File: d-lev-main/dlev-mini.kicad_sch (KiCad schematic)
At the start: 41 parts, among them J1 S6B-PH-SM4-TB, J2 S8B-PH-SM4-TB, J3 S8B-PH-SM4-TB, J4 S12B-PH-SM4-TB, U3 AMS1117-3.3

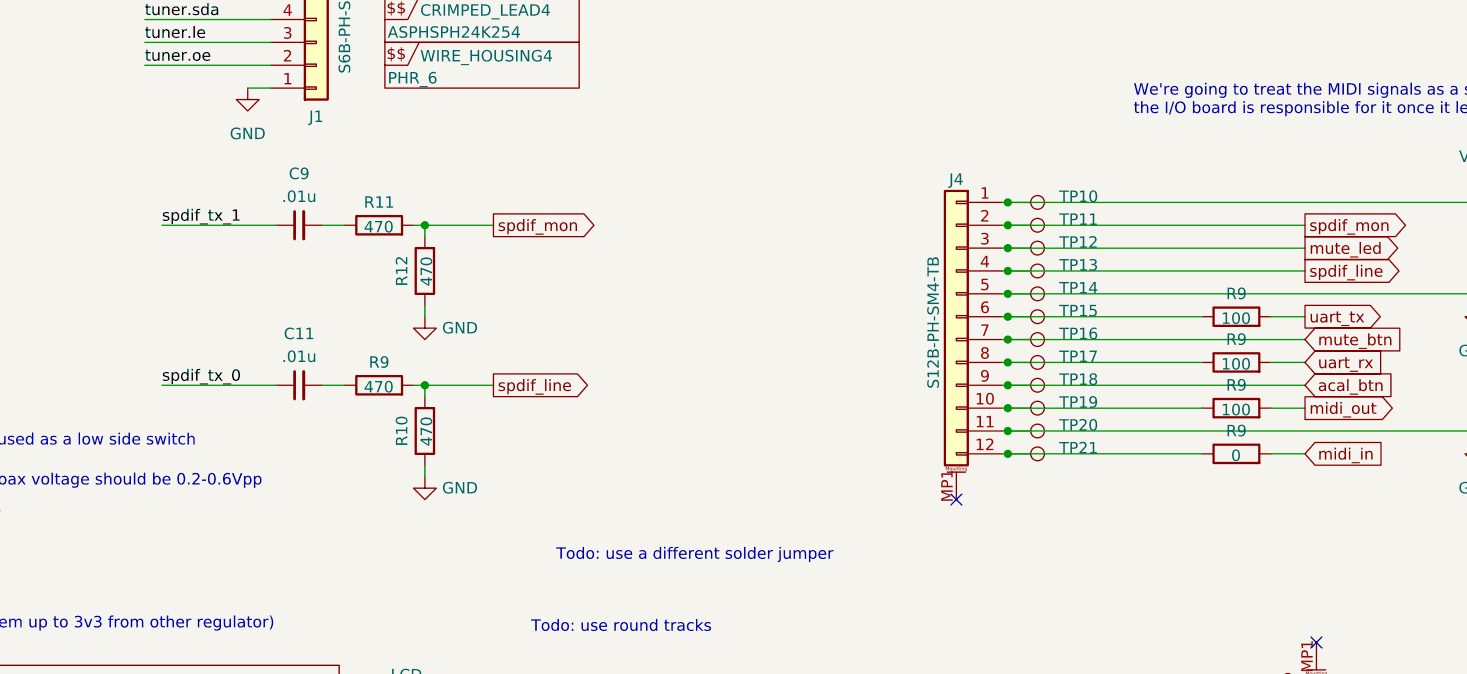
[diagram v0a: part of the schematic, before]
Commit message: many board updates
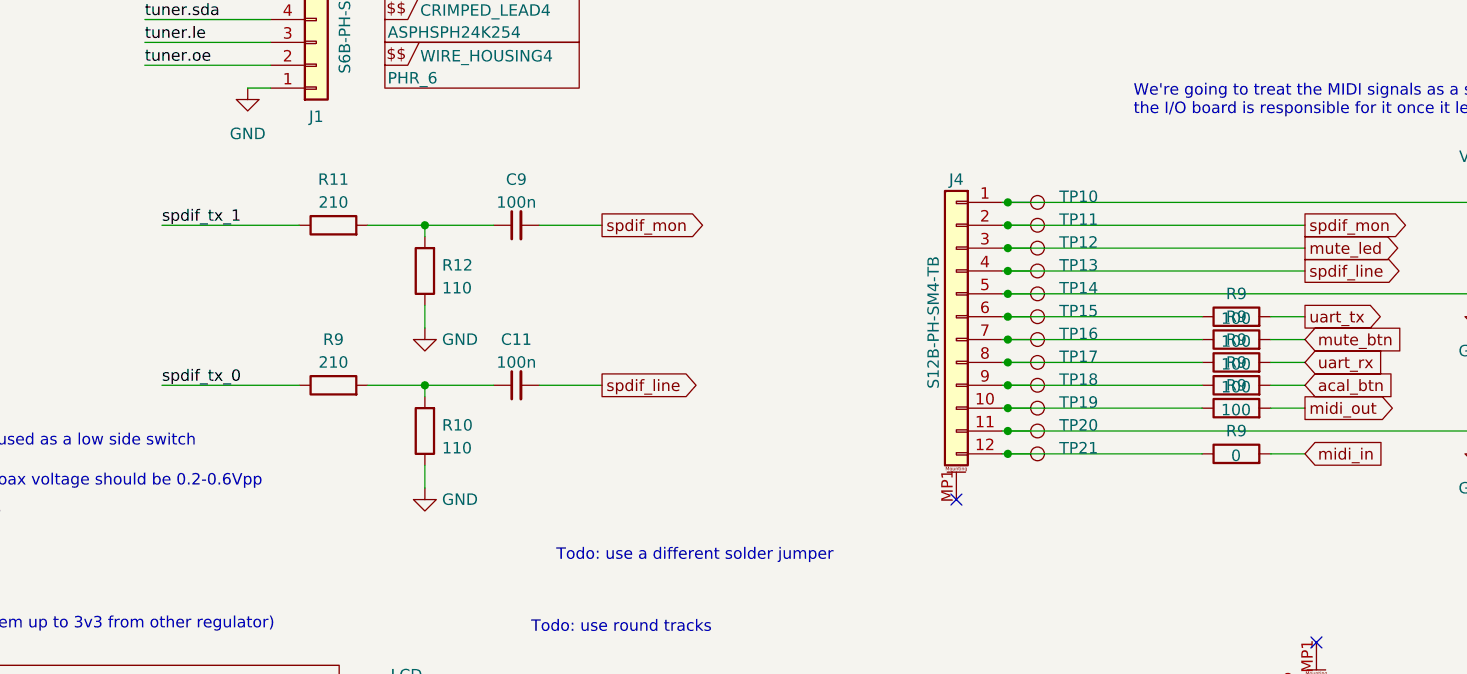
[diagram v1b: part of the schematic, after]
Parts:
- added R9 (x2): 100, Resistor_SMD:R_0603_1608Metric, symbol Device:R
- C11, C9: value .01u -> 100n
- R10, R12: value 470 -> 110
- R11, R9: value 470 -> 210
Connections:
- net acal_btn: now also R9.2; no longer J4.9 (Pin_9), TP18.1
- net mute_btn: now also R9.2; no longer J4.7 (Pin_7), TP16.1
- net spdif_line: now also C11.2; no longer R10.2, R9.2
- net spdif_mon: now also C9.2; no longer R11.2, R12.2
- net spdif_tx_0: now also R9.1; no longer C11.1
- net spdif_tx_1: now also R11.1; no longer C9.1
- new net: J4.9 (Pin_9), R9.1, TP18.1
- new net: J4.7 (Pin_7), R9.1, TP16.1
- new net: C9.1, R11.2, R12.2
- new net: C11.1, R10.2, R9.2
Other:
- moved on the sheet: C11, C9, R11, R9
